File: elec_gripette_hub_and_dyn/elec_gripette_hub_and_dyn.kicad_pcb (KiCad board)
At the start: 4 copper layers, 65 x 30 mm, 95 parts, among them J1 pico4, J2 JST EH 2, J3 Pogo-pin, J4 Dynamixel-3, J5 Dynamixel-3, J6 Pogo-pin, J7 Pogo-pin 2A, J8 Pogo-pin 2A, J9 Dynamixel-3, Q1 MMBT3906, Q2 SI2312CDS-T1-GE3, U1 FE1.1s_24-Pin_WQFN, U2 24C02S, U3 CH343P, U4 SN74LVC1G125DBV, U5 SN74LVC1G126DBVR, U6 MP2338, U7 AP63205, U8 LM5050-1, Y1 12MHz

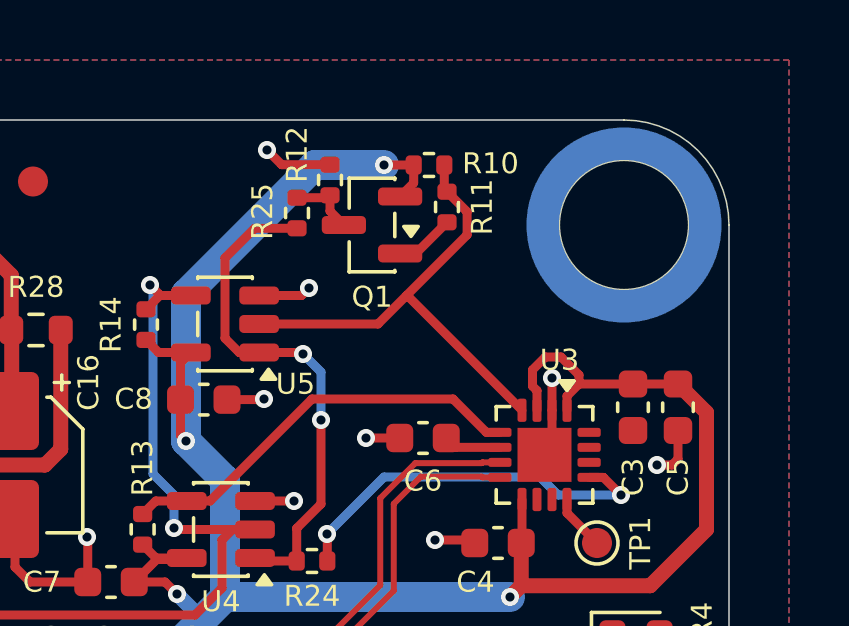
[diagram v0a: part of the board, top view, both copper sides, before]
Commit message: [update] Release A1, small batch @JLC
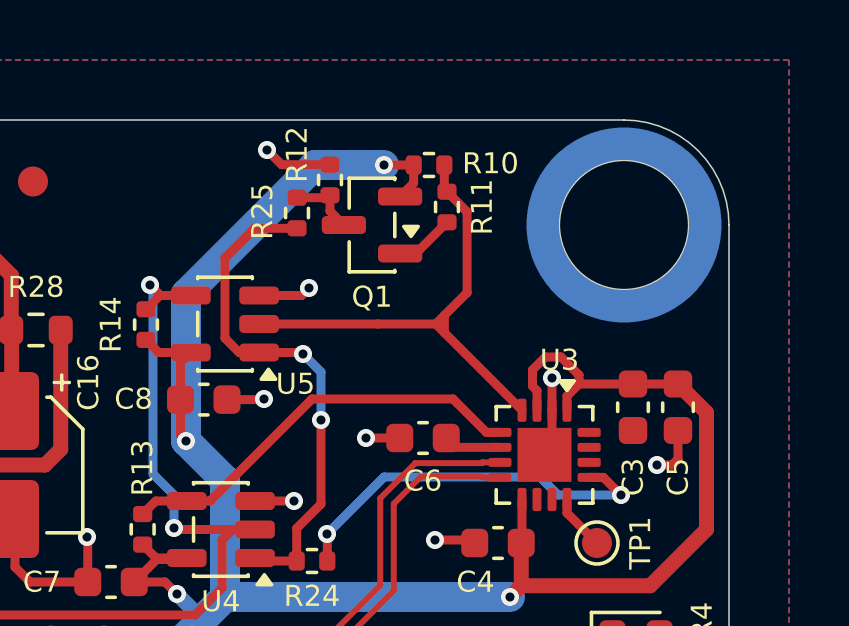
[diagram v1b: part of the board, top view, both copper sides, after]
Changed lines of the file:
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@@
 	)
 	(segment
-		(start 112.497501 54.315001)
-		(end 108.672501 50.490001)
+		(start 109.910001 51.727501)
+		(end 109.622501 51.440001)
 		(width 0.3)
 		(layer "F.Cu")
@@
 	)
 	(segment
-		(start 108.647501 50.490001)
+		(start 110.667501 47.700001)
+		(end 110.667501 50.395001)
+		(width 0.3)
+		(layer "F.Cu")
+		(net 36)
+	)
+	(segment
+		(start 109.910001 51.152501)
+		(end 109.622501 51.440001)
+		(width 0.3)
+		(layer "F.Cu")
+		(net 36)
+	)
+	(segment
+		(start 109.622501 51.440001)
 		(end 107.697501 51.440001)
 		(width 0.3)
@@
 	)
 	(segment
-		(start 110.667501 48.470001)
-		(end 108.647501 50.490001)
-		(width 0.3)
-		(layer "F.Cu")
-		(net 36)
-	)
-	(segment
-		(start 108.672501 50.490001)
-		(end 108.647501 50.490001)
+		(start 109.997501 47.030001)
+		(end 110.667501 47.700001)
 		(width 0.3)
 		(layer "F.Cu")
@@
 	)
 	(segment
-		(start 109.997501 47.030001)
-		(end 110.667501 47.700001)
+		(start 112.497501 54.315001)
+		(end 109.910001 51.727501)
 		(width 0.3)
 		(layer "F.Cu")
@@
 	)
 	(segment
-		(start 110.667501 47.700001)
-		(end 110.667501 48.470001)
+		(start 109.910001 51.152501)
+		(end 109.910001 51.727501)
 		(width 0.3)
 		(layer "F.Cu")
+		(net 36)
+	)
+	(segment
+		(start 110.667501 50.395001)
+		(end 109.910001 51.152501)
+		(width 0.3)
+		(layer "F.Cu")
